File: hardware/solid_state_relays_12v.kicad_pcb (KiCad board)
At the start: 2 copper layers, 100 x 90 mm, 88 parts, among them J1 1190297, J2 1190297, J3 1190297, J4 1190297, J5 1190297, J6 1190297, J7 1190297, J8 1190297, M1 Fan, M2 Fan, Q1 IRF4905PBF, Q2 IRF4905PBF, Q3 IRF4905PBF, Q4 IRF4905PBF, Q5 IRF4905PBF, Q6 IRF4905PBF, Q7 IRF4905PBF, Q8 IRF4905PBF

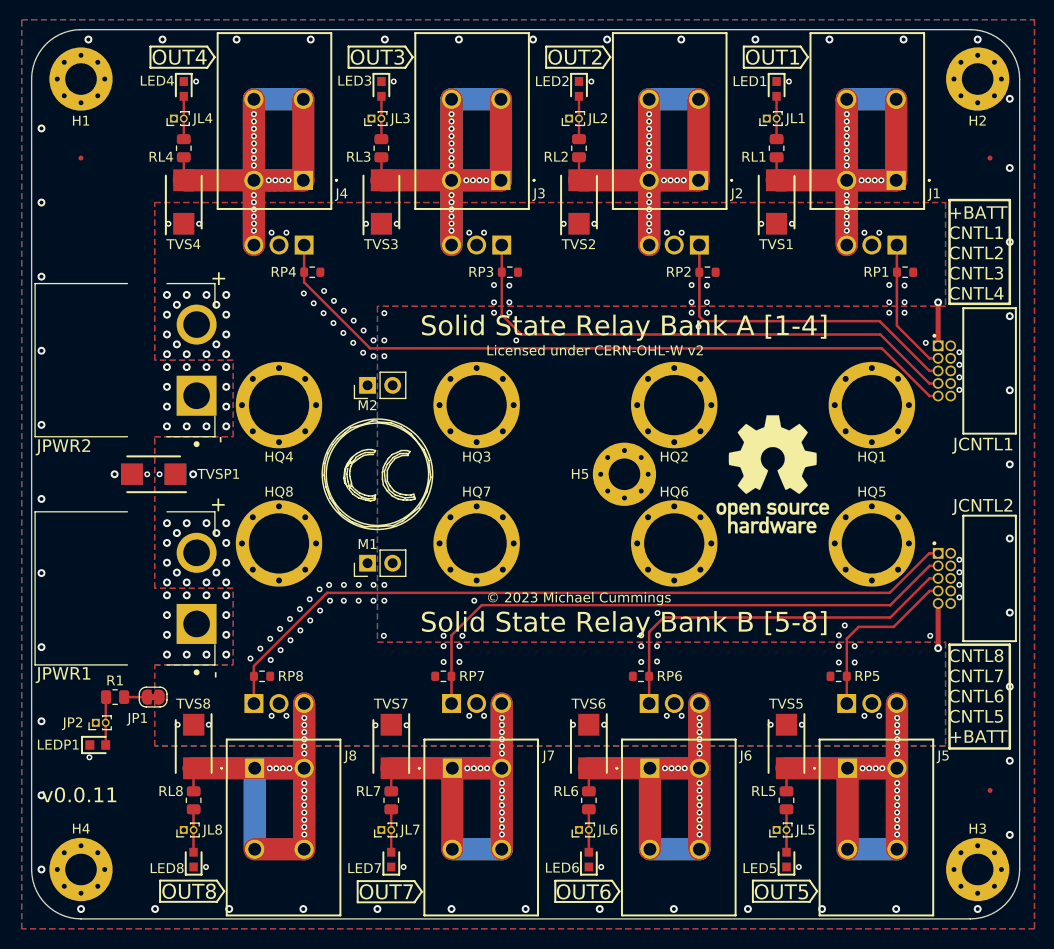
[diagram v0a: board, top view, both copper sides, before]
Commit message: Pre KiCad 7.0.0 WIP
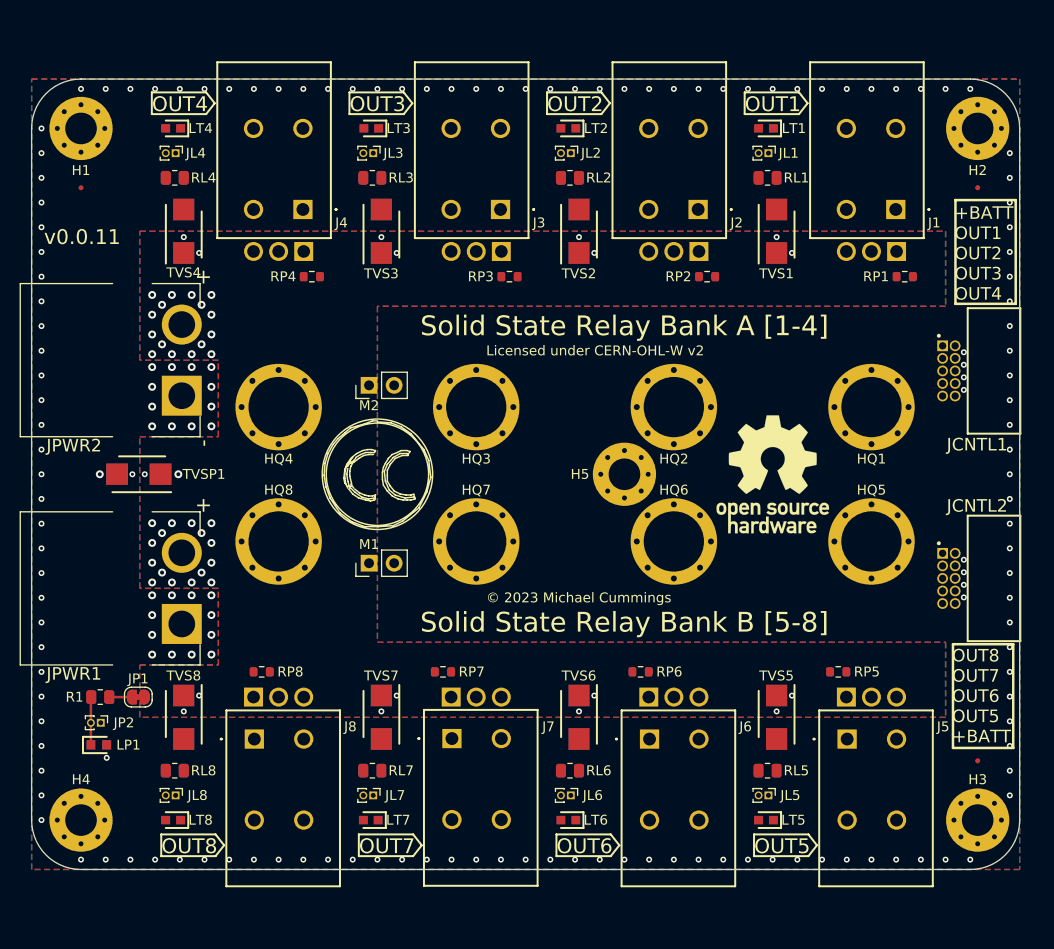
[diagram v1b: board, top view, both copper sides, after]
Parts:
- removed LED1, LED2, LED3, LED4, LED5, LED6, LED7, LED8: LTST-C190KFKT, dragon_mobile:LEDC1607X80N
- removed LEDP1: LTST-C190KGKT, dragon_mobile:LEDC1608X80N
- added LP1: LTST-C190KGKT, dragon_mobile:LEDC1608X80N, F.Cu at (21.8, 87.4)
- added LT1: LTST-C190KFKT, dragon_mobile:LEDC1607X80N, F.Cu at (89.3, 25.0)
- added LT2: LTST-C190KFKT, dragon_mobile:LEDC1607X80N, F.Cu at (69.3, 25.0)
- added LT3: LTST-C190KFKT, dragon_mobile:LEDC1607X80N, F.Cu at (49.4, 25.0)
- added LT4: LTST-C190KFKT, dragon_mobile:LEDC1607X80N, F.Cu at (29.3, 25.0)
- added LT5: LTST-C190KFKT, dragon_mobile:LEDC1607X80N, F.Cu at (89.3, 95.0)
- added LT6: LTST-C190KFKT, dragon_mobile:LEDC1607X80N, F.Cu at (69.3, 95.0)
- added LT7: LTST-C190KFKT, dragon_mobile:LEDC1607X80N, F.Cu at (49.3, 95.0)
- added LT8: LTST-C190KFKT, dragon_mobile:LEDC1607X80N, F.Cu at (29.3, 95.0)
- added OUT1: OUT1, dragon_mobile:OUT, F.Cu at (90.1, 22.4)
- added OUT2: OUT2, dragon_mobile:OUT, F.Cu at (70.1, 22.4)
- added OUT3: OUT3, dragon_mobile:OUT, F.Cu at (50.1, 22.4)
- added OUT4: OUT4, dragon_mobile:OUT, F.Cu at (30.1, 22.4)
- added OUT5: OUT5, dragon_mobile:OUT, F.Cu at (91.0, 97.5)
- added OUT6: OUT6, dragon_mobile:OUT, F.Cu at (71.0, 97.5)
- added OUT7: OUT7, dragon_mobile:OUT, F.Cu at (51.0, 97.5)
- added OUT8: OUT8, dragon_mobile:OUT, F.Cu at (31.0, 97.5)
- moved H1 5.00 mm to (20.0, 25.0)
- moved H2 5.00 mm to (110.8, 25.0)
- moved H3 5.00 mm to (110.8, 95.0)
- moved H4 5.00 mm to (20.0, 95.0)
- moved JL5 3.60 mm to (89.6, 92.5), turned to -90 degrees
- moved JL6 3.60 mm to (69.6, 92.5), turned to -90 degrees
- moved JL7 3.60 mm to (49.6, 92.5), turned to -90 degrees
- moved JL8 3.60 mm to (29.6, 92.5), turned to -90 degrees
- moved RL5 3.56 mm to (89.5, 90.0), turned to 180 degrees
- moved RL6 3.56 mm to (69.5, 90.0), turned to 180 degrees
- moved RL7 3.56 mm to (49.5, 90.0), turned to 180 degrees
- moved RL8 3.56 mm to (29.5, 90.0), turned to 180 degrees
- moved JL1 3.50 mm to (89.6, 27.5), turned to -90 degrees
- moved JL2 3.50 mm to (69.6, 27.5), turned to -90 degrees
- moved JL3 3.50 mm to (49.6, 27.5), turned to -90 degrees
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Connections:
- net /Control In - Power Out/BANK_A.CNTL1 renamed /Control In - Power Out/BANK_A.OUT1
- net /Control In - Power Out/BANK_A.CNTL2 renamed /Control In - Power Out/BANK_A.OUT2
- net /Control In - Power Out/BANK_A.CNTL3 renamed /Control In - Power Out/BANK_A.OUT3
- net /Control In - Power Out/BANK_A.CNTL4 renamed /Control In - Power Out/BANK_A.OUT4
- JCNTL2 pad 1: /Control In - Power Out/BANK_B.CNTL8 -> /Control In - Power Out/BANK_B.OUT8
- JCNTL2 pad 3: /Control In - Power Out/BANK_B.CNTL7 -> /Control In - Power Out/BANK_B.OUT7
- JCNTL2 pad 5: /Control In - Power Out/BANK_B.CNTL6 -> /Control In - Power Out/BANK_B.OUT6
- JCNTL2 pad 7: /Control In - Power Out/BANK_B.CNTL5 -> /Control In - Power Out/BANK_B.OUT5
- Q5 pad 1: /Control In - Power Out/BANK_B.CNTL5 -> /Solid State Relays - Bank B/BANK_B.OUT5
- Q6 pad 1: /Control In - Power Out/BANK_B.CNTL6 -> /Solid State Relays - Bank B/BANK_B.OUT6
- Q7 pad 1: /Control In - Power Out/BANK_B.CNTL7 -> /Solid State Relays - Bank B/BANK_B.OUT7
- Q8 pad 1: /Control In - Power Out/BANK_B.CNTL8 -> /Solid State Relays - Bank B/BANK_B.OUT8
- RP5 pad 1: /Control In - Power Out/BANK_B.CNTL5 -> /Solid State Relays - Bank B/BANK_B.OUT5
- RP6 pad 1: /Control In - Power Out/BANK_B.CNTL6 -> /Solid State Relays - Bank B/BANK_B.OUT6
- RP7 pad 1: /Control In - Power Out/BANK_B.CNTL7 -> /Solid State Relays - Bank B/BANK_B.OUT7
- RP8 pad 1: /Control In - Power Out/BANK_B.CNTL8 -> /Solid State Relays - Bank B/BANK_B.OUT8
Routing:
- net /Control In - Power Out/BANK_B.CNTL8: track 77.8 -> 0.00 mm
- net /Control In - Power Out/BANK_A.OUT4: track 72.7 -> 0.00 mm
- net OUT4: track 62.1 -> 0.00 mm, vias 18 -> 0
- net OUT3: track 62.1 -> 0.00 mm, vias 18 -> 0
- net OUT2: track 62.1 -> 0.00 mm, vias 18 -> 0
- net OUT1: track 62.1 -> 0.00 mm, vias 18 -> 0
- net OUT8: track 61.2 -> 0.00 mm, vias 18 -> 0
- net OUT7: track 61.2 -> 0.00 mm, vias 18 -> 0
- net OUT6: track 61.2 -> 0.00 mm, vias 18 -> 0
- net OUT5: track 61.2 -> 0.00 mm, vias 18 -> 0
- net /Control In - Power Out/BANK_B.CNTL7: track 59.1 -> 0.00 mm
- net /Control In - Power Out/BANK_A.OUT3: track 54.1 -> 0.00 mm
- net /Control In - Power Out/BANK_B.CNTL6: track 38.7 -> 0.00 mm
- net /Control In - Power Out/BANK_A.OUT2: track 33.7 -> 0.00 mm
- net /Control In - Power Out/BANK_B.CNTL5: track 17.8 -> 0.00 mm
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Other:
- board size 100 x 90 mm -> 100 x 80 mm
- board text added: "+BATT OUT1 OUT2 OUT3 OUT4"
- board text added: "OUT8 OUT7 OUT6 OUT5 +BATT"
- board text removed: "+BATT CNTL1 CNTL2 CNTL3 CNTL4"
- board text removed: "CNTL8 CNTL7 CNTL6 CNTL5 +BATT"
- board text removed: "JPWR1"
- board text removed: "JPWR2"
- board text removed: "OUT1"
- board text removed: "OUT2"
- board text removed: "OUT3"
- board text removed: "OUT4"
- board text removed: "OUT5"
- board text removed: "OUT6"
- board text removed: "OUT7"
- board text removed: "OUT8"
